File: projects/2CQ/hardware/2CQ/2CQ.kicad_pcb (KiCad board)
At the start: 4 copper layers, 48.5 x 111 mm, 17 parts, among them SW1 TOGGLE_ON-ON, U1 ES_DAISY_PATCH_SM_REV1

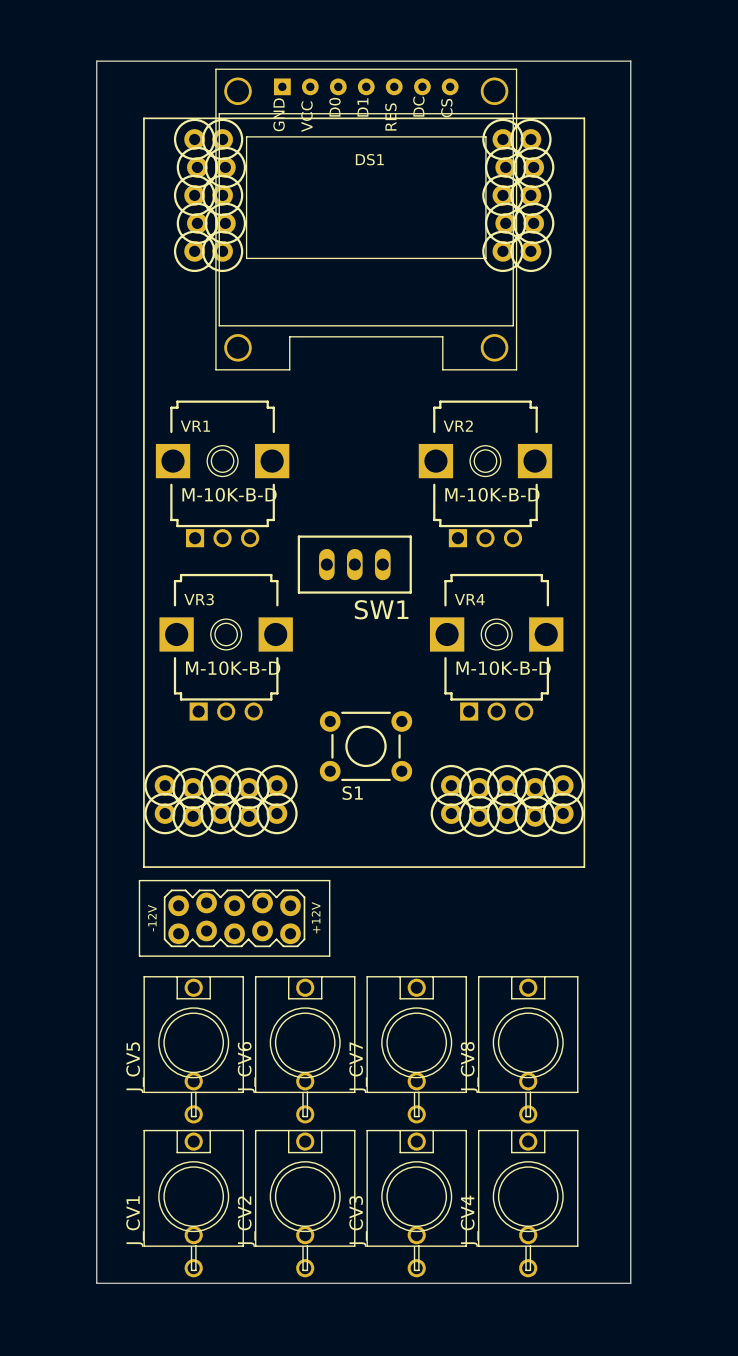
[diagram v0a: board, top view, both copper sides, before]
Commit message: Moving shit around
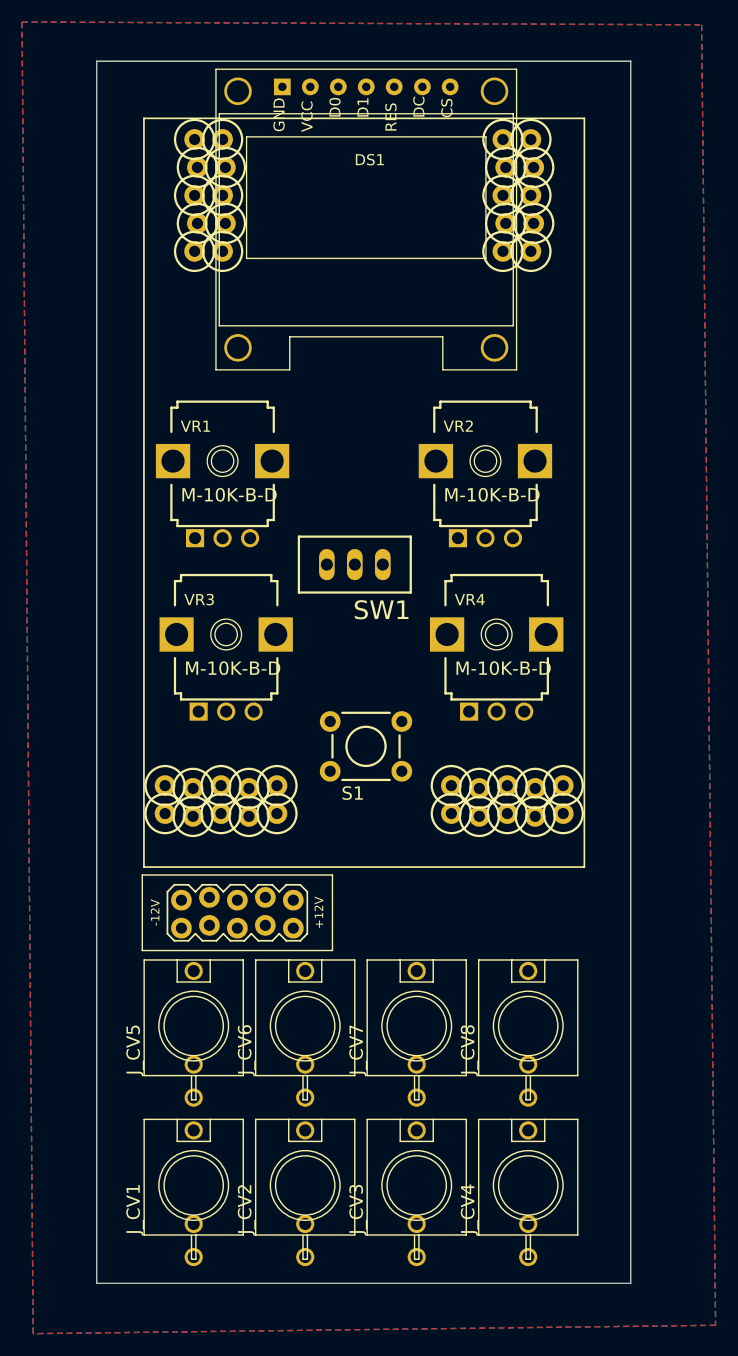
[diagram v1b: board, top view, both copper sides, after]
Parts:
- moved J_CV5 1.52 mm to (82.4, 132.1)
- moved J_CV6 1.52 mm to (92.5, 132.1)
- moved J_CV7 1.52 mm to (102.6, 132.1)
- moved J_CV8 1.52 mm to (112.8, 132.1)
- moved J_CV1 1.02 mm to (82.4, 146.6)
- moved J_CV2 1.02 mm to (92.5, 146.6)
- moved J_CV3 1.02 mm to (102.6, 146.6)
- moved J_CV4 1.02 mm to (112.8, 146.6)
- moved EP1 0.57 mm to (86.4, 121.8)
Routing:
- added copper zone on B.Cu, net GND
- added copper zone on F.Cu, net GND
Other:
- copper layers 4 -> 2
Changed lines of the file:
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@@
 	(layers
 		(0 "F.Cu" signal "Front")
-		(1 "In1.Cu" signal)
-		(2 "In2.Cu" signal)
 		(31 "B.Cu" signal "Back")
 		(34 "B.Paste" user)
@@
 			(layer "dielectric 1"
 				(type "core")
-				(thickness 0.480066)
-				(material "FR4")
-				(epsilon_r 4.5)
-				(loss_tangent 0.02)
-			)
-			(layer "In1.Cu"
-				(type "copper")
-				(thickness 0.035)
-			)
-			(layer "dielectric 2"
-				(type "prepreg")
-				(thickness 0.480066)
-				(material "FR4")
-				(epsilon_r 4.5)
-				(loss_tangent 0.02)
-			)
-			(layer "In2.Cu"
-				(type "copper")
-				(thickness 0.035)
-			)
-			(layer "dielectric 3"
-				(type "core")
-				(thickness 0.480066)
+				(thickness 1.510198)
 				(material "FR4")
 				(epsilon_r 4.5)
@@
 	(footprint "ES_Daisy_Patch_SM_FB_Rev1:S_JACK"
 		(layer "F.Cu")
-		(at 92.522 133.604)
+		(at 92.522 132.08)
 		(property "Reference" "J_CV6"
 			(at -4.7498 4.4704 90)
@@
 	(footprint "ES_Daisy_Patch_SM_FB_Rev1:S_JACK"
 		(layer "F.Cu")
-		(at 102.649 147.574)
+		(at 102.649 146.558)
 		(property "Reference" "J_CV3"
 			(at -4.7498 4.4704 90)
@@
 	(footprint "ES_Daisy_Patch_SM_FB_Rev1:S_JACK"
 		(layer "F.Cu")
-		(at 102.649 133.604)
+		(at 102.649 132.08)
 		(property "Reference" "J_CV7"
 			(at -4.7498 4.4704 90)
@@
 	(footprint "ES_Daisy_Patch_SM_FB_Rev1:S_JACK"
 		(layer "F.Cu")
-		(at 82.395 133.604)
+		(at 82.395 132.08)
 		(property "Reference" "J_CV5"
 			(at -4.7498 4.4704 90)
@@
 	(footprint "ES_Daisy_Patch_SM_FB_Rev1:S_JACK"
 		(layer "F.Cu")
-		(at 82.395 147.574)
+		(at 82.395 146.558)
 		(property "Reference" "J_CV1"
 			(at -4.7498 4.4704 90)
@@
 	(footprint "ES_Daisy_Patch_SM_FB_Rev1:S_JACK"
 		(layer "F.Cu")
-		(at 112.776 147.574)
+		(at 112.776 146.558)
 		(property "Reference" "J_CV4"
 			(at -4.7498 4.4704 90)
@@
 	(footprint "ES_Daisy_Patch_SM_FB_Rev1:EURORACK_POWER_SHROUD_LOCK"
 		(layer "F.Cu")
-		(at 86.106 122.301 180)
+		(at 86.36 121.793 180)
 		(property "Reference" "EP1"
 			(at 0 0 360)
@@
 			(size 2.5 2.5)
 			(drill 2)
-			(layers "F&B.Cu" "*.Mask")
+			(layers "*.Cu" "*.Mask")
 		)
 		(pad "" np_thru_hole circle
@@
 			(size 2.5 2.5)
 			(drill 2)
-			(layers "F&B.Cu" "*.Mask")
+			(layers "*.Cu" "*.Mask")
 		)
 		(pad "" np_thru_hole circle
@@
 			(size 2.5 2.5)
 			(drill 2)
-			(layers "F&B.Cu" "*.Mask")
+			(layers "*.Cu" "*.Mask")
 		)
 		(pad "" np_thru_hole circle
@@
 			(size 2.5 2.5)
 			(drill 2)
-			(layers "F&B.Cu" "*.Mask")
+			(layers "*.Cu" "*.Mask")
 		)
 		(pad "1" thru_hole rect
@@
 	(footprint "ES_Daisy_Patch_SM_FB_Rev1:S_JACK"
 		(layer "F.Cu")
-		(at 92.522 147.574)
+		(at 92.522 146.558)
 		(property "Reference" "J_CV2"
 			(at -4.7498 4.4704 90)
@@
 	(footprint "ES_Daisy_Patch_SM_FB_Rev1:S_JACK"
 		(layer "F.Cu")
-		(at 112.776 133.604)
+		(at 112.776 132.08)
 		(property "Reference" "J_CV8"
 			(at -4.7498 4.4704 90)
@@
 		)
 	)
+	(zone
+		(net 2)
+		(net_name "GND")
+		(layers "F&B.Cu")
+		(hatch edge 0.5)
+		(connect_pads
+			(clearance 0.5)
+		)
+		(min_thickness 0.25)
+		(filled_areas_thickness no)
+		(fill yes
+			(thermal_gap 0.5)
+			(thermal_bridge_width 0.5)
+		)
+		(polygon
+			(pts
+				(xy 66.802 40.894) (xy 128.524 41.148) (xy 129.794 159.258) (xy 67.818 160.02)
+			)
+		)
+	)
